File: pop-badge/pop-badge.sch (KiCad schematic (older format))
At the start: 1 part, among them J1 Conn_01x04

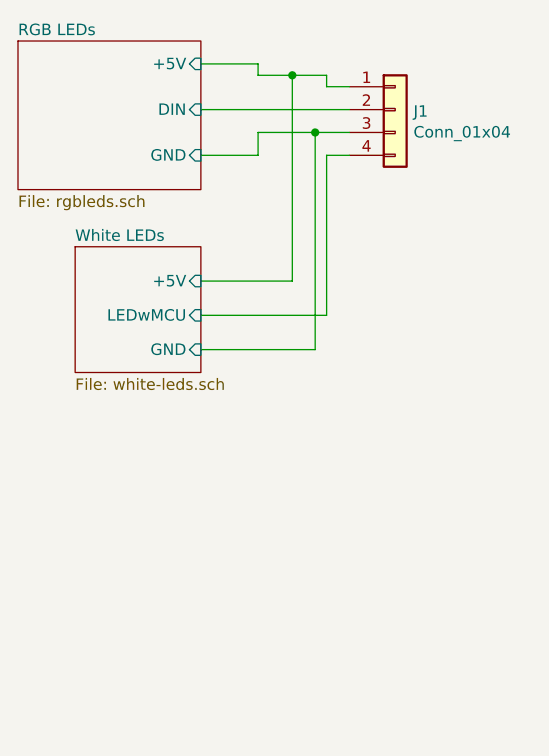
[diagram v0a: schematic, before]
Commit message: much more layouting
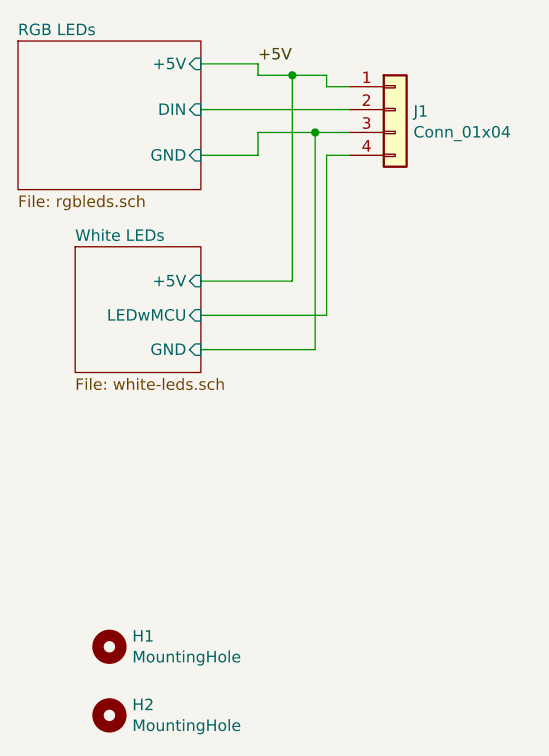
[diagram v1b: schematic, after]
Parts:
- added H1, H2: MountingHole, MountingHole:MountingHole_4.3mm_M4, symbol Mechanical:MountingHole
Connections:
- net RGB LEDs/+5V renamed +5V
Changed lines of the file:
@@
 Wire Wire Line
 	2150 2450 1900 2450
+$Comp
+L Mechanical:MountingHole H1
+U 1 1 6190E265
+P 1500 5000
+F 0 "H1" H 1600 5046 50  0000 L CNN
+F 1 "MountingHole" H 1600 4955 50  0000 L CNN
+F 2 "MountingHole:MountingHole_4.3mm_M4" H 1500 5000 50  0001 C CNN
+F 3 "~" H 1500 5000 50  0001 C CNN
+	1    1500 5000
+	1    0    0    -1
+$EndComp
+$Comp
+L Mechanical:MountingHole H2
+U 1 1 6190E4B0
+P 1500 5300
+F 0 "H2" H 1600 5346 50  0000 L CNN
+F 1 "MountingHole" H 1600 5255 50  0000 L CNN
+F 2 "MountingHole:MountingHole_4.3mm_M4" H 1500 5300 50  0001 C CNN
+F 3 "~" H 1500 5300 50  0001 C CNN
+	1    1500 5300
+	1    0    0    -1
+$EndComp
+Text Label 2150 2450 0    50   ~ 0
++5V
 $EndSCHEMATC

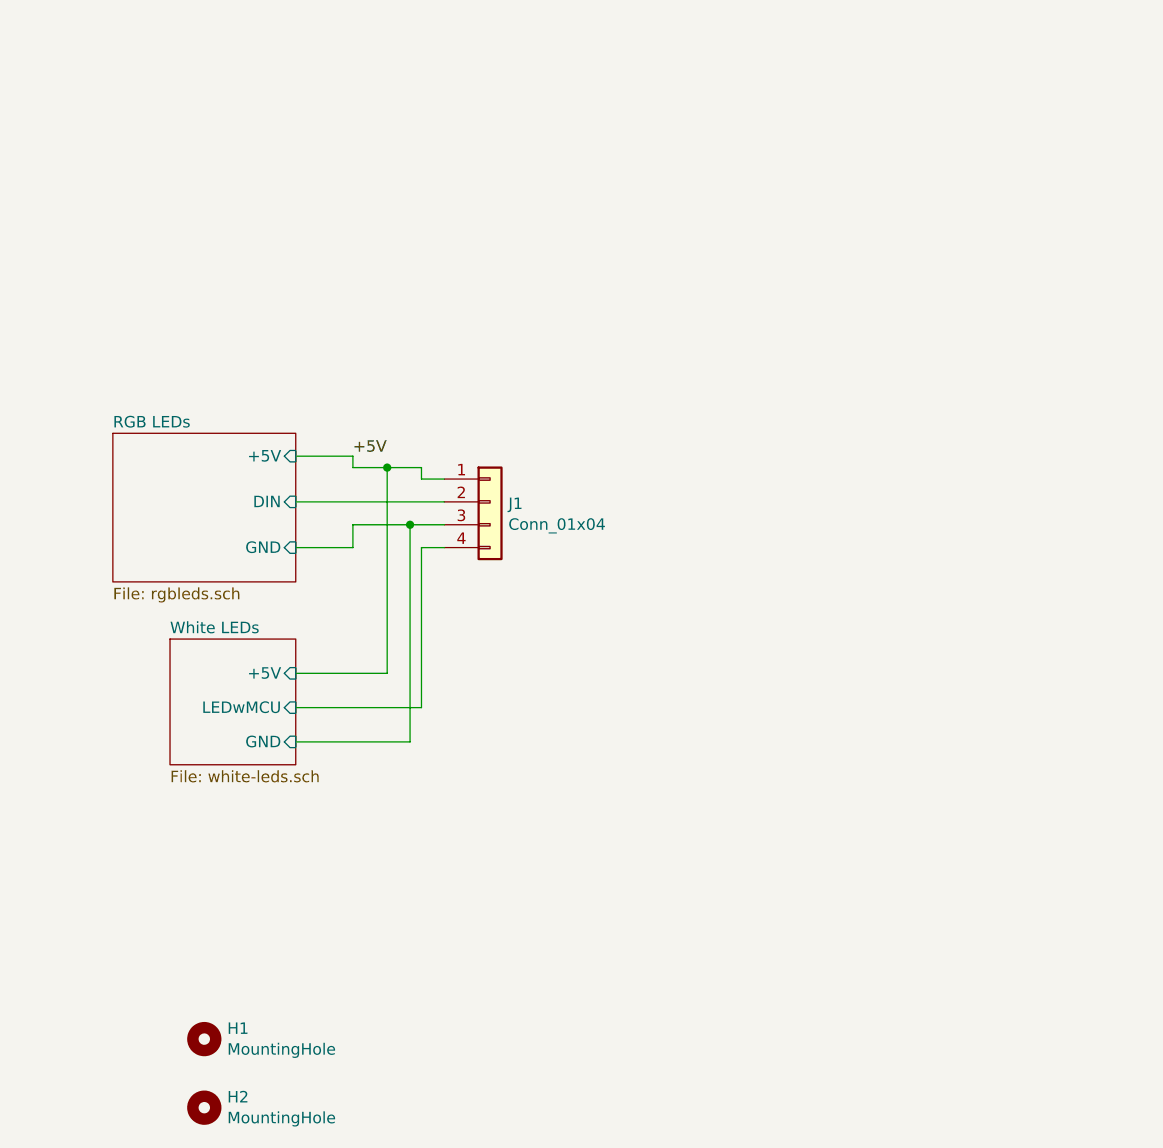
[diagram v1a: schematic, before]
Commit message: routing done
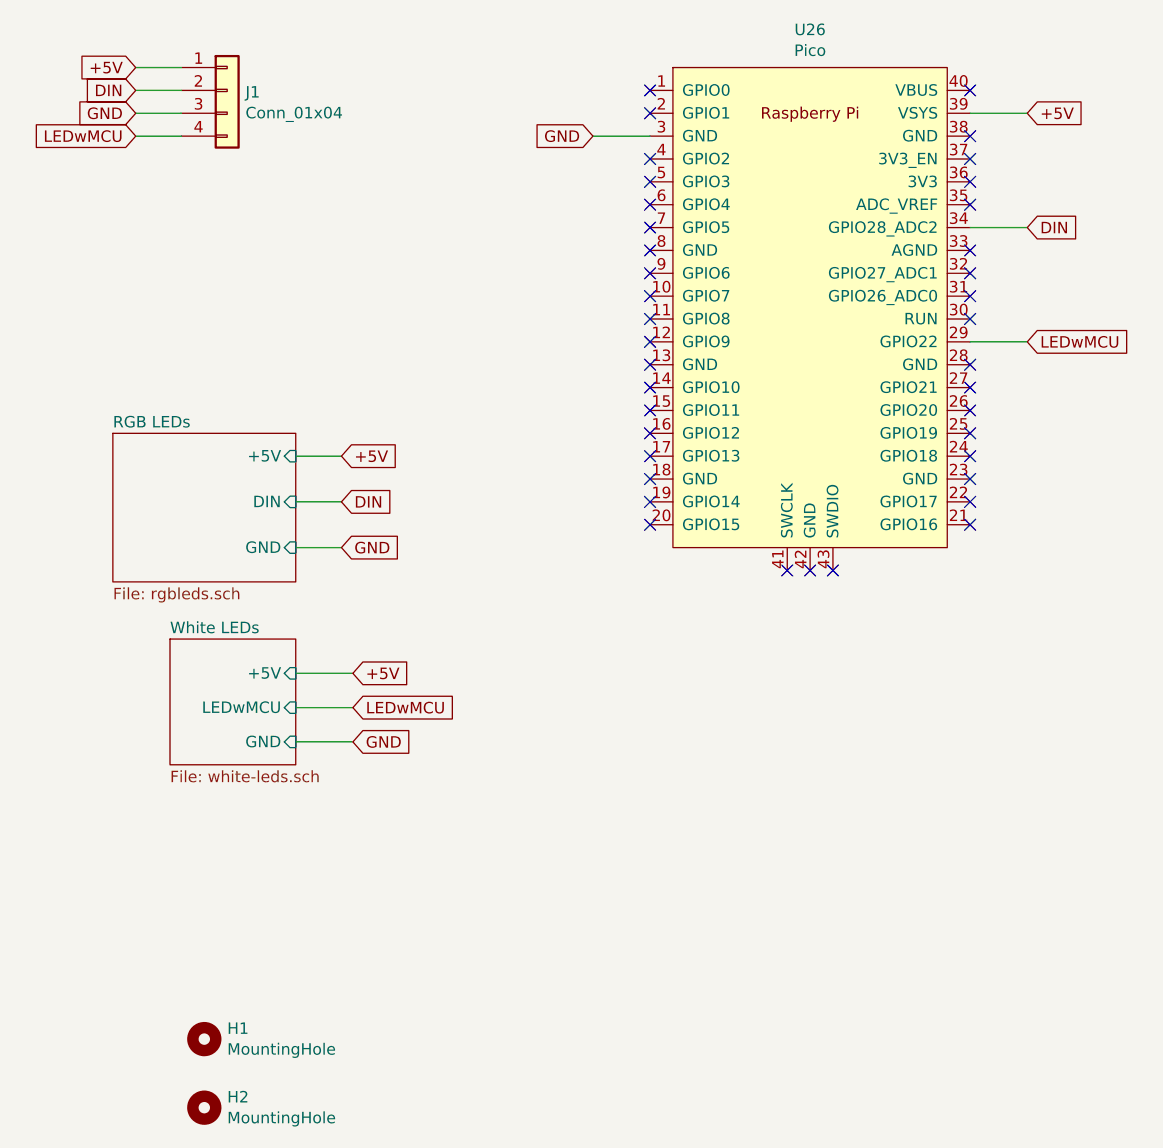
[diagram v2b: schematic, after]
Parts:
- added U26: Pico, RPi_Pico:RPi_Pico_SMD, symbol RPi-Pico:Pico
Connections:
- net +5V: now also U26.39 (VSYS)
- net RGB LEDs/DIN renamed DIN
- net DIN: now also U26.34 (GPIO28_ADC2)
- net RGB LEDs/GND renamed GND
- net GND: now also U26.3 (GND)
- net White LEDs/LEDwMCU renamed LEDwMCU
- net LEDwMCU: now also U26.29 (GPIO22)
- no-connect marks 0 -> 39
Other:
- moved on the sheet: J1
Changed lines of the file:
@@
 Comment4 ""
 $EndDescr
-Wire Wire Line
-	2150 2500 2300 2500
-Wire Wire Line
-	2550 2550 2450 2550
-Wire Wire Line
-	2450 2550 2450 2500
-$Sheet
-S 1350 3250 550  550
-U 615492B8
-F0 "White LEDs" 50
-F1 "white-leds.sch" 50
-F2 "LEDwMCU" I R 1900 3550 50
-F3 "GND" I R 1900 3700 50
-F4 "+5V" I R 1900 3400 50
-$EndSheet
 $Comp
 L Connector_Generic:Conn_01x04 J1
 U 1 1 6163BF0A
-P 2750 2650
-F 0 "J1" H 2830 2642 50  0000 L CNN
-F 1 "Conn_01x04" H 2830 2551 50  0000 L CNN
-F 2 "Connector_PinHeader_1.27mm:PinHeader_1x04_P1.27mm_Vertical" H 2750 2650 50  0001 C CNN
-F 3 "~" H 2750 2650 50  0001 C CNN
-	1    2750 2650
+P 1600 850
+F 0 "J1" H 1680 842 50  0000 L CNN
+F 1 "Conn_01x04" H 1680 751 50  0000 L CNN
+F 2 "Connector_PinHeader_1.27mm:PinHeader_1x04_P1.27mm_Vertical" H 1600 850 50  0001 C CNN
+F 3 "~" H 1600 850 50  0001 C CNN
+	1    1600 850
 	1    0    0    -1
 $EndComp
-Wire Wire Line
-	2550 2750 2400 2750
-Wire Wire Line
-	2450 2850 2550 2850
-Wire Wire Line
-	2450 2850 2450 3550
-Wire Wire Line
-	1900 3550 2450 3550
-Wire Wire Line
-	1900 3700 2400 3700
-Connection ~ 2400 2750
-Wire Wire Line
-	2400 2750 2150 2750
-Wire Wire Line
-	2400 3700 2400 2750
-Wire Wire Line
-	2300 2500 2300 3400
-Wire Wire Line
-	2300 3400 1900 3400
-Connection ~ 2300 2500
-Wire Wire Line
-	2300 2500 2450 2500
 $Sheet
 S 1100 2350 800  650
@@
 F4 "DIN" I R 1900 2650 50
 $EndSheet
-Wire Wire Line
-	2150 2750 2150 2850
-Wire Wire Line
-	2150 2850 1900 2850
-Wire Wire Line
-	1900 2650 2550 2650
-Wire Wire Line
-	2150 2500 2150 2450
-Wire Wire Line
-	2150 2450 1900 2450
 $Comp
 L Mechanical:MountingHole H1
@@
 	1    0    0    -1
 $EndComp
-Text Label 2150 2450 0    50   ~ 0
+$Comp
+L RPi-Pico:Pico U26
+U 1 1 61A68EB5
+P 4150 1800
+F 0 "U26" H 4150 3015 50  0000 C CNN
+F 1 "Pico" H 4150 2924 50  0000 C CNN
+F 2 "RPi_Pico:RPi_Pico_SMD" V 4150 1800 50  0001 C CNN
+F 3 "" H 4150 1800 50  0001 C CNN
+	1    4150 1800
+	1    0    0    -1
+$EndComp
+NoConn ~ 4050 2950
+NoConn ~ 4150 2950
+NoConn ~ 4250 2950
+NoConn ~ 4850 2650
+NoConn ~ 4850 2550
+NoConn ~ 4850 2450
+NoConn ~ 4850 2350
+NoConn ~ 4850 2250
+NoConn ~ 4850 2150
+NoConn ~ 4850 2050
+NoConn ~ 4850 2750
+NoConn ~ 4850 1850
+NoConn ~ 4850 1750
+NoConn ~ 4850 1650
+NoConn ~ 4850 1550
+NoConn ~ 4850 1350
+NoConn ~ 4850 1250
+NoConn ~ 4850 1150
+NoConn ~ 4850 1050
+NoConn ~ 4850 850
+NoConn ~ 3450 850
+NoConn ~ 3450 950
+NoConn ~ 3450 1150
+NoConn ~ 3450 1250
+NoConn ~ 3450 1350
+NoConn ~ 3450 1450
+NoConn ~ 3450 1550
+NoConn ~ 3450 1650
+NoConn ~ 3450 1750
+NoConn ~ 3450 1850
+NoConn ~ 3450 1950
+NoConn ~ 3450 2050
+NoConn ~ 3450 2150
+NoConn ~ 3450 2250
+NoConn ~ 3450 2350
+NoConn ~ 3450 2450
+NoConn ~ 3450 2550
+NoConn ~ 3450 2650
+NoConn ~ 3450 2750
+Text GLabel 1200 1050 0    50   Input ~ 0
+LEDwMCU
+Text GLabel 5100 950  2    50   Input ~ 0
 +5V
+Text GLabel 5100 1450 2    50   Input ~ 0
+DIN
+Text GLabel 3200 1050 0    50   Input ~ 0
+GND
+$Sheet
+S 1350 3250 550  550
+U 615492B8
+F0 "White LEDs" 50
+F1 "white-leds.sch" 50
+F2 "LEDwMCU" I R 1900 3550 50
+F3 "GND" I R 1900 3700 50
+F4 "+5V" I R 1900 3400 50
+$EndSheet
+Wire Wire Line
+	1400 1050 1200 1050
+Wire Wire Line
+	3200 1050 3450 1050
+Wire Wire Line
+	4850 1450 5100 1450
+Wire Wire Line
+	5100 950  4850 950
+Text GLabel 2150 3400 2    50   Input ~ 0
++5V
+Text GLabel 2150 3550 2    50   Input ~ 0
+LEDwMCU
+Text GLabel 2150 3700 2    50   Input ~ 0
+GND
+Wire Wire Line
+	2150 3700 1900 3700
+Wire Wire Line
+	1900 3550 2150 3550
+Wire Wire Line
+	2150 3400 1900 3400
+Text GLabel 5100 1950 2    50   Input ~ 0
+LEDwMCU
+Wire Wire Line
+	5100 1950 4850 1950
+Wire Wire Line
+	1200 950  1400 950
+Wire Wire Line
+	1400 850  1200 850
+Wire Wire Line
+	1200 750  1400 750
+Text GLabel 1200 950  0    50   Input ~ 0
+GND
+Text GLabel 1200 850  0    50   Input ~ 0
+DIN
+Text GLabel 1200 750  0    50   Input ~ 0
++5V
+Text GLabel 2100 2450 2    50   Input ~ 0
++5V
+Text GLabel 2100 2650 2    50   Input ~ 0
+DIN
+Text GLabel 2100 2850 2    50   Input ~ 0
+GND
+Wire Wire Line
+	2100 2450 1900 2450
+Wire Wire Line
+	1900 2650 2100 2650
+Wire Wire Line
+	2100 2850 1900 2850
 $EndSCHEMATC
